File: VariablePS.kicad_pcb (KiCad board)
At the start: 2 copper layers, 60 x 40 mm, 17 parts, among them J1 VOUT, J2 VIN, U1 LM317T

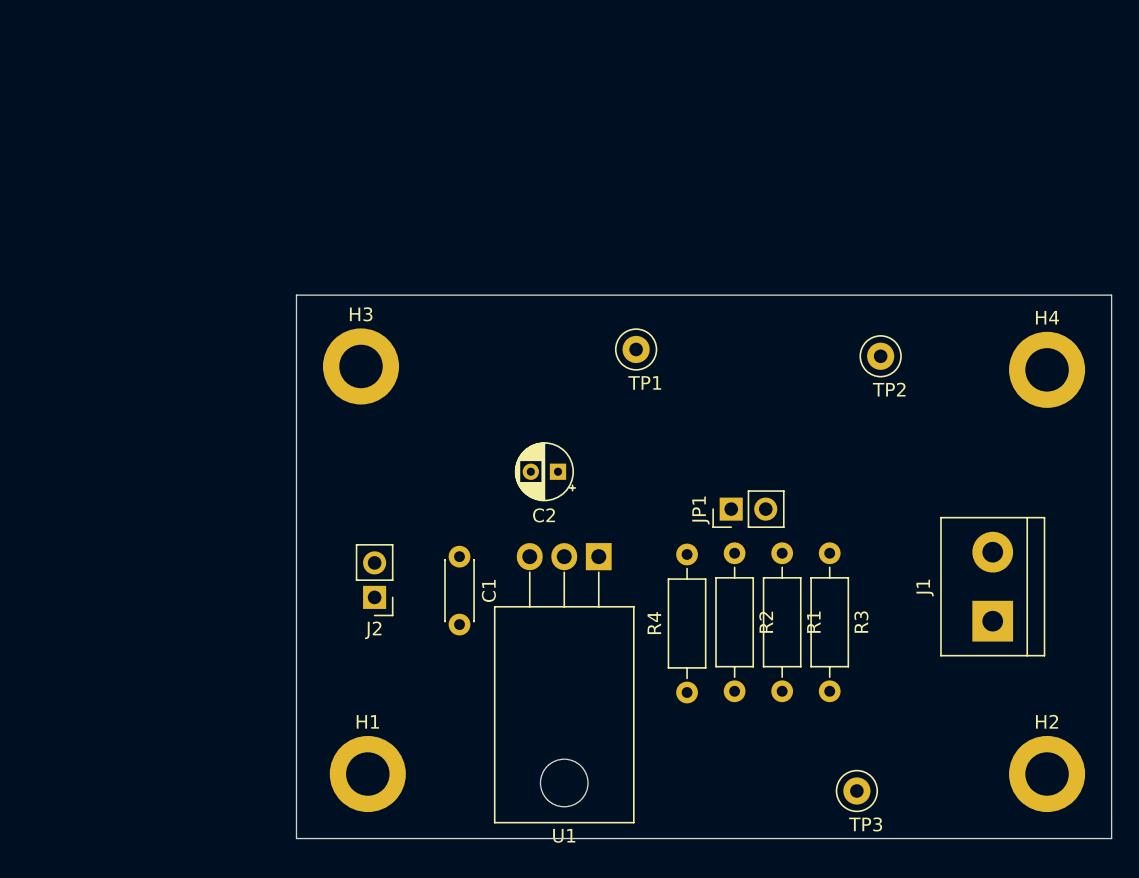
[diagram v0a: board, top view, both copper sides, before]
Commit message: PCB routing done, gerber files generated (v1.0).
Signed-off-by: Ion Bold <bold.ion86@gmail.com>
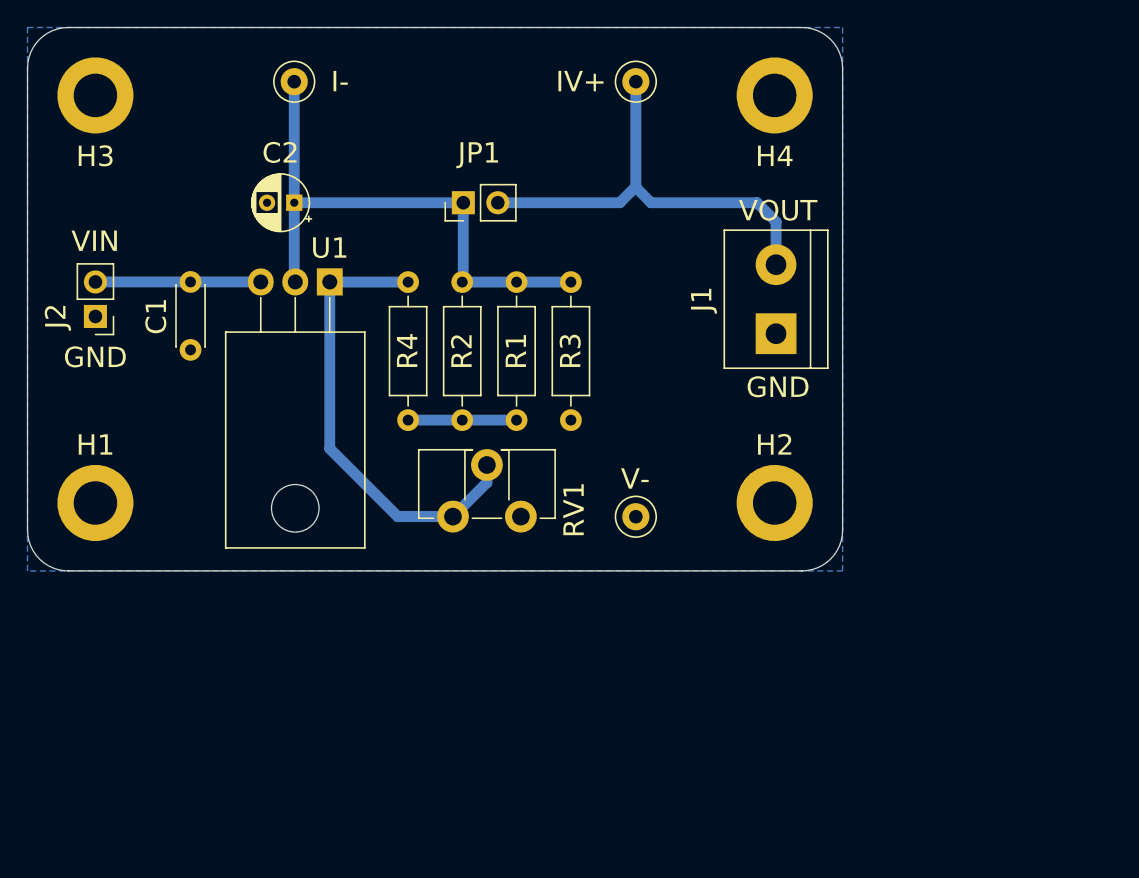
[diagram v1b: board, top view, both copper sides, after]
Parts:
- removed TP1: I-, TestPoint:TestPoint_Loop_D1.80mm_Drill1.0mm_Beaded
- added I-: I-, TestPoint:TestPoint_Loop_D1.80mm_Drill1.0mm_Beaded, F.Cu at (99.8, 44.3)
- added RV1: 1k, Potentiometer_THT:Potentiometer_ACP_CA9-H3,8_Horizontal, F.Cu at (111.5, 76.3)
- moved JP1 30.0 mm to (112.3, 53.2)
- moved J2 29.2 mm to (85.2, 61.6)
- moved R4 28.7 mm to (108.2, 69.2)
- moved H4 28.5 mm to (135.2, 45.3)
- moved C1 28.3 mm to (92.2, 59.0)
- moved U1 28.3 mm to (102.5, 59.0)
- moved R2 28.3 mm to (112.2, 59.0)
- moved H2 28.3 mm to (135.2, 75.3)
- moved H1 28.3 mm to (85.2, 75.3)
- moved R1 27.9 mm to (116.2, 59.0)
- moved H3 27.9 mm to (85.2, 45.3)
- moved C2 27.7 mm to (99.8, 53.2)
- moved R3 27.6 mm to (120.2, 59.0)
- moved IV+ 27.1 mm to (125.0, 44.3)
- moved J1 26.5 mm to (135.3, 62.8)
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- renumbered TP2 to IV+, TP3 to V-
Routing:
- net Net-(C2-Pad1): track 0.00 -> 41.1 mm
- net Net-(R4-Pad2): track 0.00 -> 34.0 mm
- net Net-(J1-Pad2): track 0.00 -> 33.0 mm
- net Net-(C1-Pad1): track 0.00 -> 12.2 mm
- net Net-(R1-Pad2): track 0.00 -> 7.98 mm
- added copper zone on B.Cu, net GND
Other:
- outline, holes or cut-outs redrawn
- board text added: "GND"
- board text added: "VIN"
- board text added: "VOUT"
